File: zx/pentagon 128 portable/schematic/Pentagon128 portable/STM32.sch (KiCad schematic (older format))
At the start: 0 parts

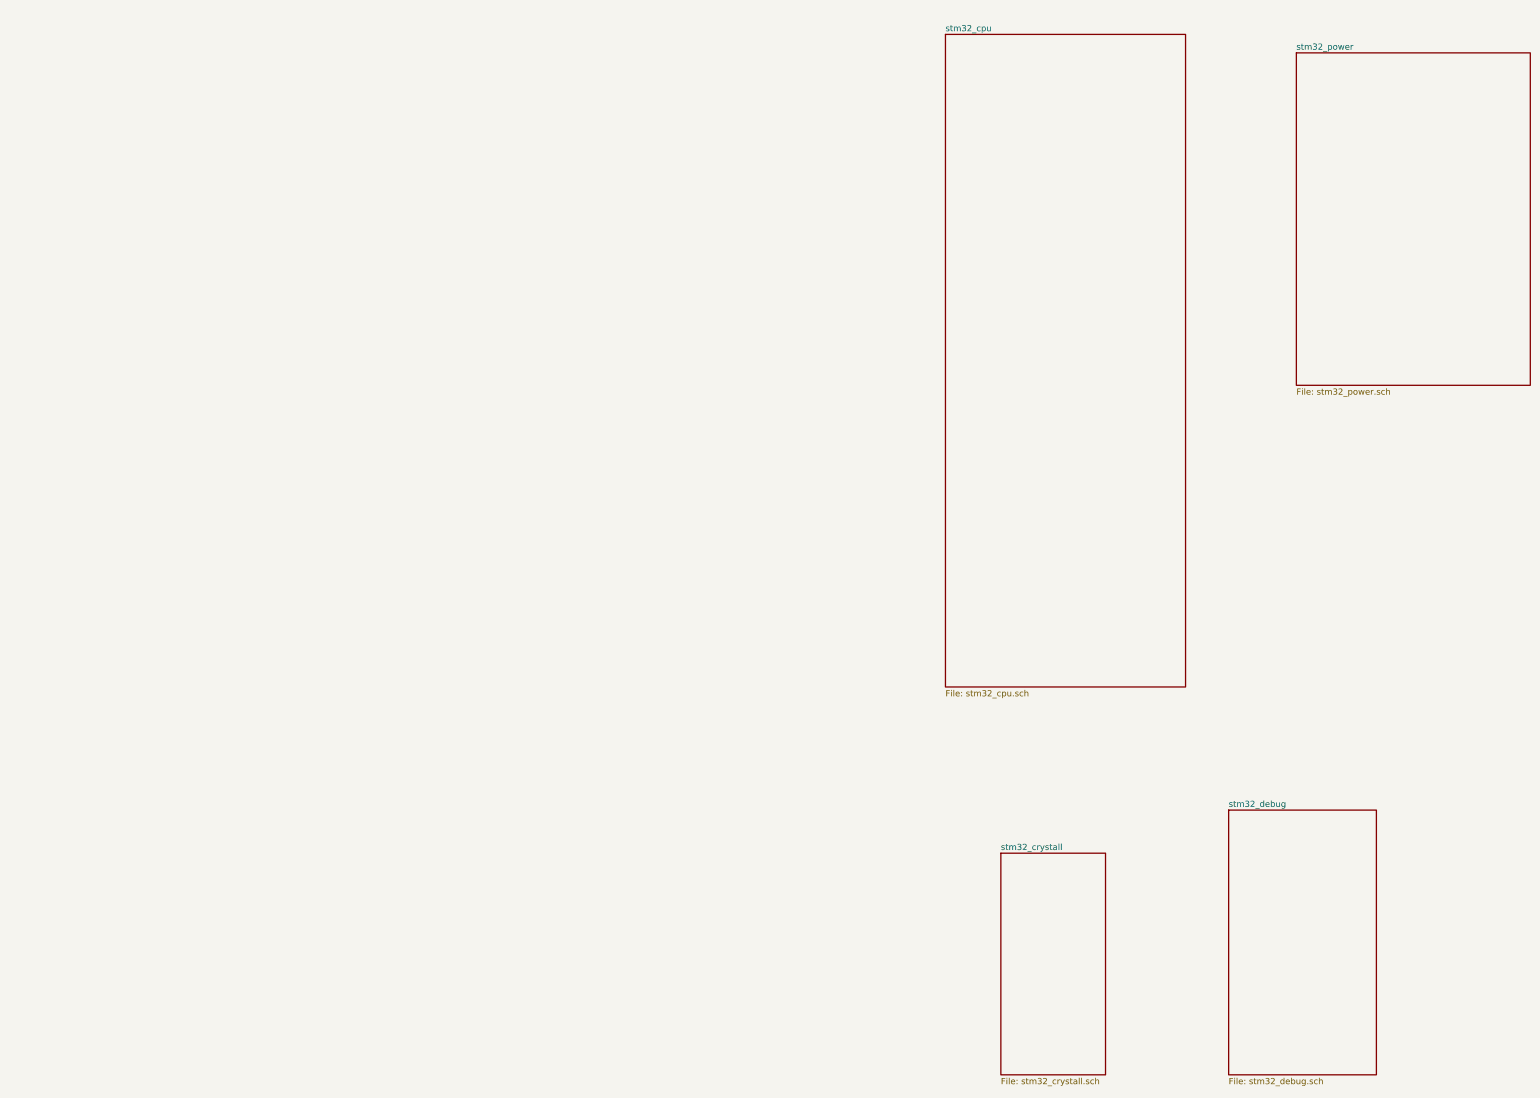
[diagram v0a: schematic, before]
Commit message: updated schemes
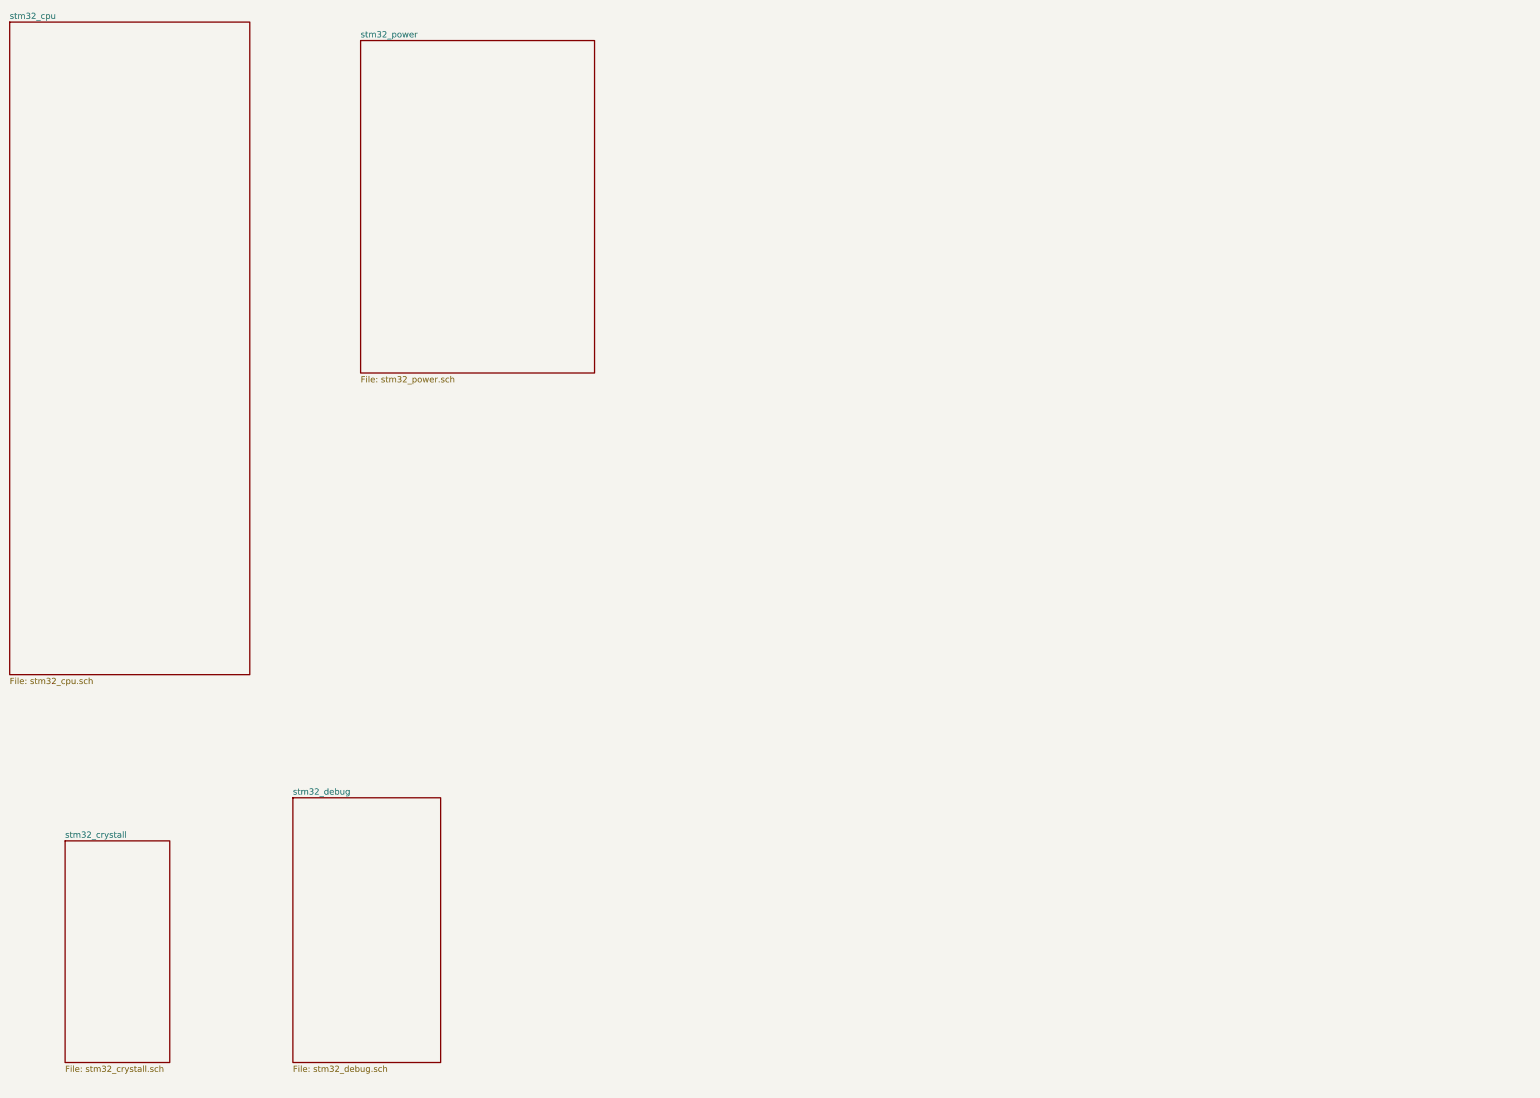
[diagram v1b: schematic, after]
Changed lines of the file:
@@
 $EndDescr
 $Sheet
-S 9500 1150 1950 5300
+S 1900 1050 1950 5300
 U 5F7467A7
 F0 "stm32_cpu" 50
@@
 $EndSheet
 $Sheet
-S 12350 1300 1900 2700
+S 4750 1200 1900 2700
 U 5F747225
 F0 "stm32_power" 50
@@
 $EndSheet
 $Sheet
-S 9950 7800 850  1800
+S 2350 7700 850  1800
 U 5F8C0463
 F0 "stm32_crystall" 50
@@
 $EndSheet
 $Sheet
-S 11800 7450 1200 2150
+S 4200 7350 1200 2150
 U 5F98BCEA
 F0 "stm32_debug" 50
